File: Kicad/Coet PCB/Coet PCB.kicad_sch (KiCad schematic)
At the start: 5 parts, among them U1 BNO055 Stemma, U2 Teensy4.1, U3 BMP280 Stemma, U4 MP1584EN, U5 XL4015_DC

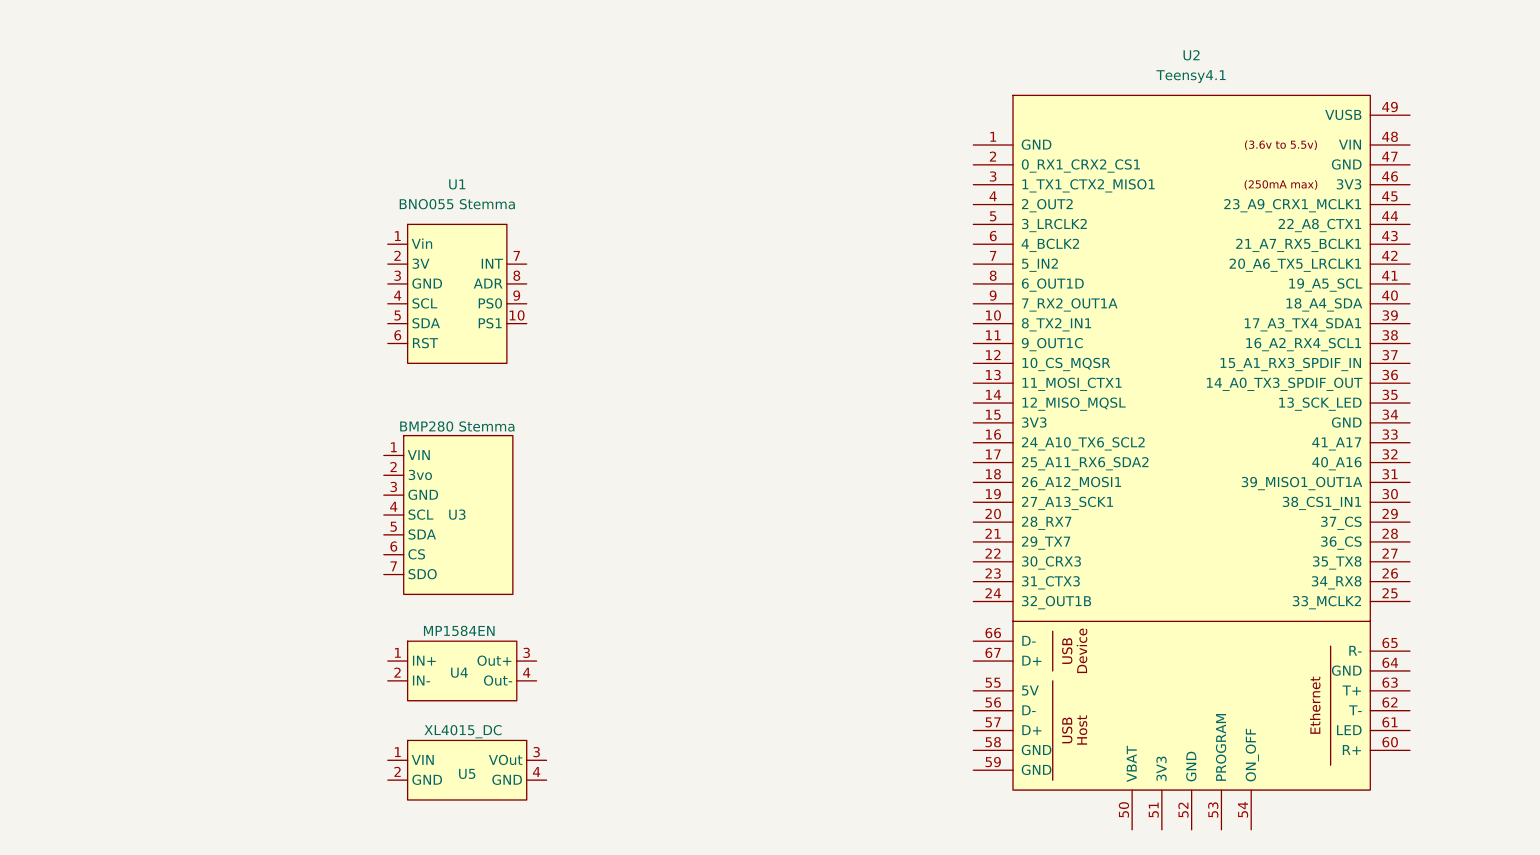
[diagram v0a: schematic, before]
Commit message: He acabat les conecions del esquema!
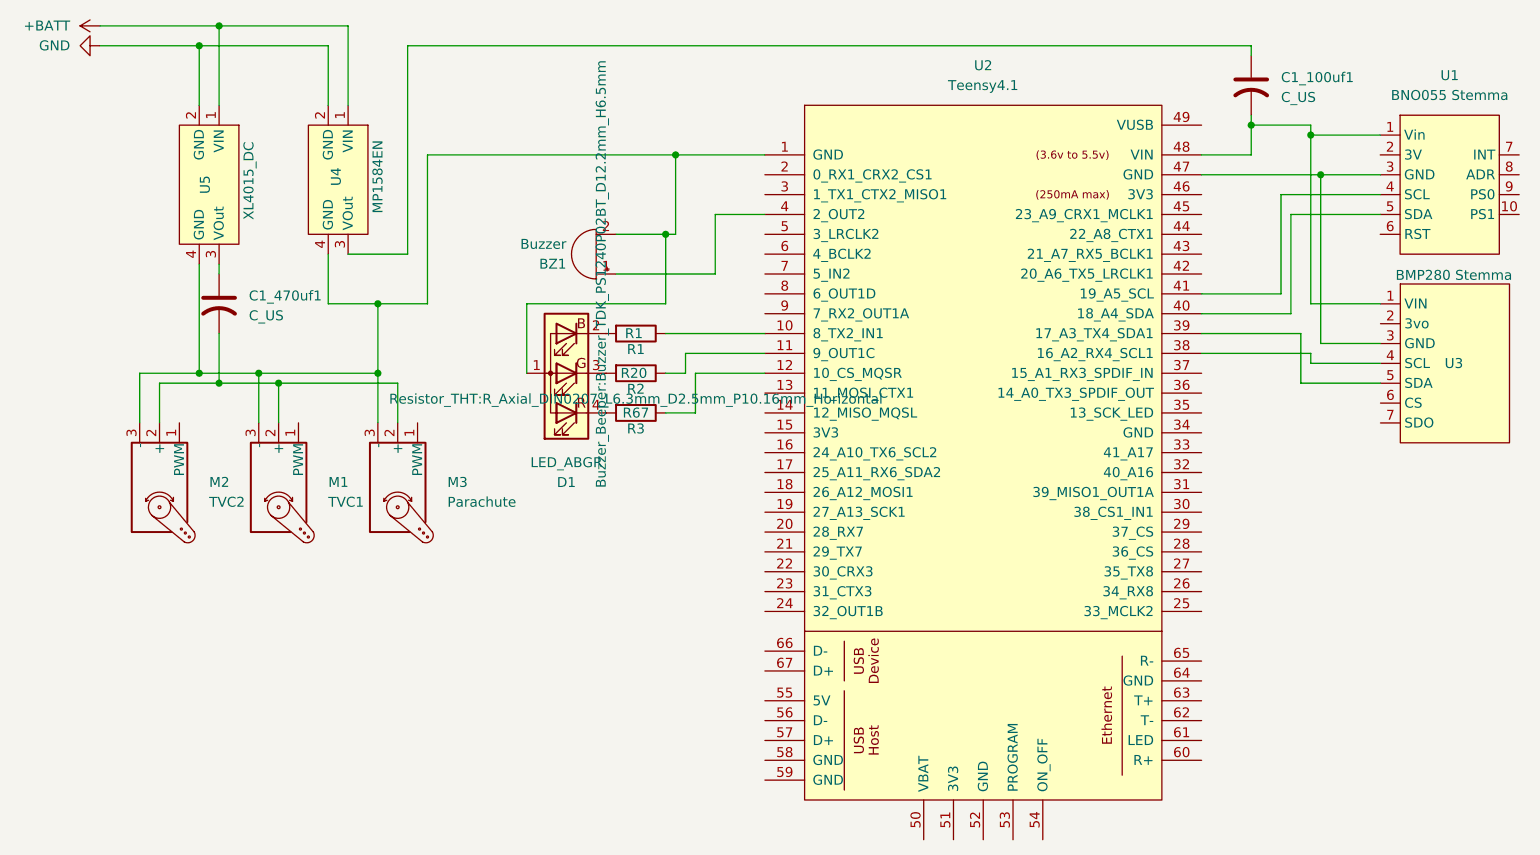
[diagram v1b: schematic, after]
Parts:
- added BZ1: Buzzer, Buzzer_Beeper:Buzzer_TDK_PS1240P02BT_D12.2mm_H6.5mm, symbol Device:Buzzer
- added C1_100uf1, C1_470uf1: C_US, Capacitor_SMD:CP_Elec_8x5.4, symbol Device:C_US
- added D1: LED_ABGR, LED_THT:LED_D5.0mm-4_RGB_Wide_Pins, symbol Device:LED_ABGR
- added M1: TVC1, Connector_PinHeader_1.00mm:PinHeader_1x03_P1.00mm_Vertical, symbol Motor:Motor_Servo
- added M2: TVC2, Connector_PinHeader_1.00mm:PinHeader_1x03_P1.00mm_Vertical, symbol Motor:Motor_Servo
- added M3: Parachute, Connector_PinHeader_1.00mm:PinHeader_1x03_P1.00mm_Vertical, symbol Motor:Motor_Servo
- added R1: R1, Resistor_THT:R_Axial_DIN0207_L6.3mm_D2.5mm_P10.16mm_Horizontal, symbol Device:R
- added R2: R20, Resistor_THT:R_Axial_DIN0207_L6.3mm_D2.5mm_P10.16mm_Horizontal, symbol Device:R
- added R3: R67, Resistor_THT:R_Axial_DIN0207_L6.3mm_D2.5mm_P10.16mm_Horizontal, symbol Device:R
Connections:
- net +BATT: now reaches U5.1 (VIN)
- net +BATT: now also U4.1 (VIN)
- net GND: now reaches U5.2 (GND)
- net GND: now also U4.2 (GND)
- net at U5.3 (VOut): now also C1_470uf1.1
- net at U5.4 (GND): now also U2.1 (GND), U4.4 (GND), BZ1.2 (-), D1.1 (A), M1.3 (-), M2.3 (-), M3.3 (-)
- net at U4.3 (VOut): now also C1_100uf1.1
- net at U1.1 (Vin): now also U2.48 (VIN), C1_100uf1.2
- net at U1.3 (GND): now also U2.47 (GND)
- net at U1.4 (SCL): now also U2.41 (19_A5_SCL)
- net at U1.5 (SDA): now also U2.40 (18_A4_SDA)
- net at U2.10 (8_TX2_IN1): now also R1.1
- net at U2.11 (9_OUT1C): now also R2.1
- net at U2.12 (10_CS_MQSR): now also R3.1
- net at U2.4 (2_OUT2): now also BZ1.1 (+)
- new net: C1_470uf1.2, M1.2 (+), M2.2 (+), M3.2 (+)
- new net: D1.3 (GK), R2.2
- new net: D1.2 (BK), R1.2
- new net: D1.4 (RK), R3.2
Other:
- moved on the sheet: U1, U2, U5
